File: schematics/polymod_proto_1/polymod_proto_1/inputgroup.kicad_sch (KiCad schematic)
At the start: 10 parts, among them J13 Conn_01x08_Male, U13 74LS165

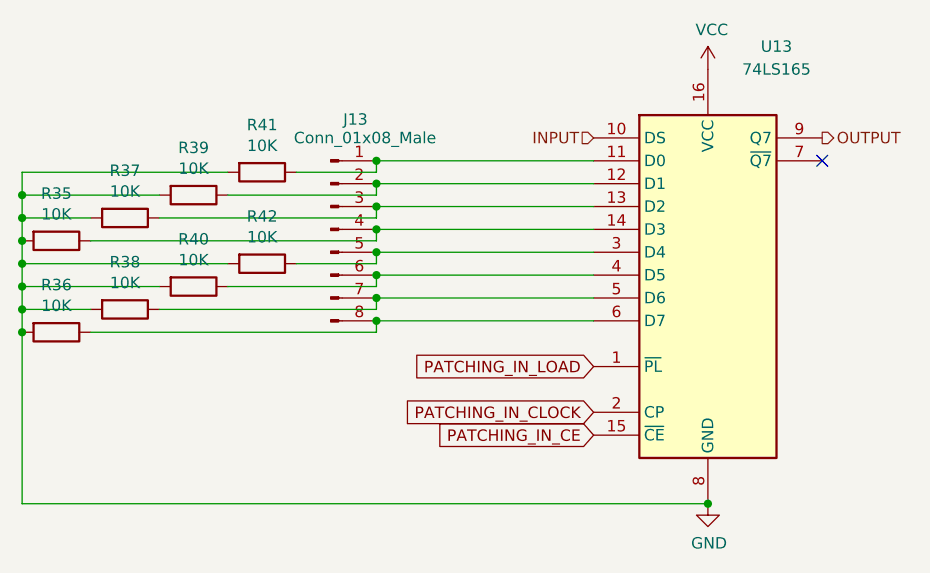
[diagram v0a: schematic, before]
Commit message: routing started
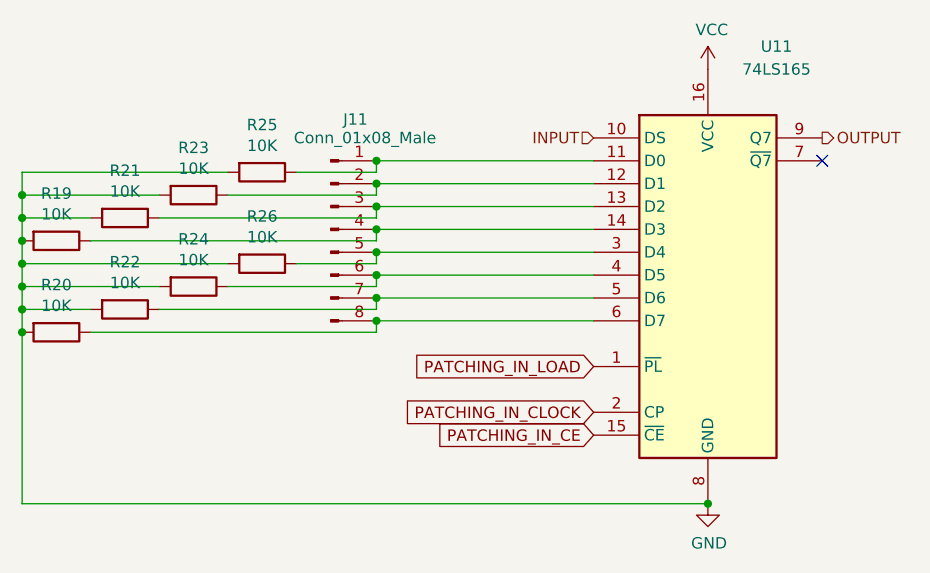
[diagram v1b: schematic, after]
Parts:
- renumbered J13 to J11, R35 to R19, R36 to R20, R37 to R21, R38 to R22, R39 to R23, R40 to R24, R41 to R25, R42 to R26, U13 to U11
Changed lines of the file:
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@@
   (symbol (lib_id "Device:R") (at 118.11 91.44 270)
     (in_bom yes) (on_board yes)
-    (property "Reference" "R40" (id 0) (at 118.11 86.1822 90))
+    (property "Reference" "R24" (id 0) (at 118.11 86.1822 90))
     (property "Value" "10K" (id 1) (at 118.11 88.4936 90))
     (property "Footprint" "Resistor_SMD:R_0805_2012Metric" (id 2) (at 118.11 89.662 90)
@@
   (symbol (lib_id "74xx:74LS165") (at 175.26 90.17 0)
     (in_bom yes) (on_board yes)
-    (property "Reference" "U13" (id 0) (at 182.88 64.77 0))
+    (property "Reference" "U11" (id 0) (at 182.88 64.77 0))
     (property "Value" "74LS165" (id 1) (at 182.88 67.31 0))
     (property "Footprint" "Package_SO:SOIC-16_3.9x9.9mm_P1.27mm" (id 2) (at 175.26 90.17 0)
@@
   (symbol (lib_id "Connector:Conn_01x08_Male") (at 133.35 85.09 0)
     (in_bom yes) (on_board yes)
-    (property "Reference" "J13" (id 0) (at 136.0932 72.8726 0))
+    (property "Reference" "J11" (id 0) (at 136.0932 72.8726 0))
     (property "Value" "Conn_01x08_Male" (id 1) (at 137.16 74.93 0))
     (property "Footprint" "Connector_PinSocket_2.54mm:PinSocket_1x08_P2.54mm_Vertical" (id 2) (at 133.35 85.09 0)
@@
   (symbol (lib_id "power:VCC") (at 175.26 67.31 0)
     (in_bom yes) (on_board yes)
-    (property "Reference" "#PWR030" (id 0) (at 175.26 71.12 0)
+    (property "Reference" "#PWR026" (id 0) (at 175.26 71.12 0)
       (effects (font (size 1.27 1.27)) hide)
     )
@@
   (symbol (lib_id "Device:R") (at 102.87 96.52 270)
     (in_bom yes) (on_board yes)
-    (property "Reference" "R36" (id 0) (at 102.87 91.2622 90))
+    (property "Reference" "R20" (id 0) (at 102.87 91.2622 90))
     (property "Value" "10K" (id 1) (at 102.87 93.5736 90))
     (property "Footprint" "Resistor_SMD:R_0805_2012Metric" (id 2) (at 102.87 94.742 90)
@@
   (symbol (lib_id "Device:R") (at 102.87 86.36 270)
     (in_bom yes) (on_board yes)
-    (property "Reference" "R35" (id 0) (at 102.87 81.1022 90))
+    (property "Reference" "R19" (id 0) (at 102.87 81.1022 90))
     (property "Value" "10K" (id 1) (at 102.87 83.4136 90))
     (property "Footprint" "Resistor_SMD:R_0805_2012Metric" (id 2) (at 102.87 84.582 90)
@@
   (symbol (lib_id "Device:R") (at 118.11 81.28 270)
     (in_bom yes) (on_board yes)
-    (property "Reference" "R39" (id 0) (at 118.11 76.0222 90))
+    (property "Reference" "R23" (id 0) (at 118.11 76.0222 90))
     (property "Value" "10K" (id 1) (at 118.11 78.3336 90))
     (property "Footprint" "Resistor_SMD:R_0805_2012Metric" (id 2) (at 118.11 79.502 90)
@@
   (symbol (lib_id "Device:R") (at 110.49 83.82 270)
     (in_bom yes) (on_board yes)
-    (property "Reference" "R37" (id 0) (at 110.49 78.5622 90))
+    (property "Reference" "R21" (id 0) (at 110.49 78.5622 90))
     (property "Value" "10K" (id 1) (at 110.49 80.8736 90))
     (property "Footprint" "Resistor_SMD:R_0805_2012Metric" (id 2) (at 110.49 82.042 90)
@@
   (symbol (lib_id "Device:R") (at 125.73 88.9 270)
     (in_bom yes) (on_board yes)
-    (property "Reference" "R42" (id 0) (at 125.73 83.6422 90))
+    (property "Reference" "R26" (id 0) (at 125.73 83.6422 90))
     (property "Value" "10K" (id 1) (at 125.73 85.9536 90))
     (property "Footprint" "Resistor_SMD:R_0805_2012Metric" (id 2) (at 125.73 87.122 90)
@@
   (symbol (lib_id "Device:R") (at 125.73 78.74 270)
     (in_bom yes) (on_board yes)
-    (property "Reference" "R41" (id 0) (at 125.73 73.4822 90))
+    (property "Reference" "R25" (id 0) (at 125.73 73.4822 90))
     (property "Value" "10K" (id 1) (at 125.73 75.7936 90))
     (property "Footprint" "Resistor_SMD:R_0805_2012Metric" (id 2) (at 125.73 76.962 90)
@@
   (symbol (lib_id "power:GND") (at 175.26 115.57 0)
     (in_bom yes) (on_board yes)
-    (property "Reference" "#PWR031" (id 0) (at 175.26 121.92 0)
+    (property "Reference" "#PWR027" (id 0) (at 175.26 121.92 0)
       (effects (font (size 1.27 1.27)) hide)
     )
@@
   (symbol (lib_id "Device:R") (at 110.49 93.98 270)
     (in_bom yes) (on_board yes)
-    (property "Reference" "R38" (id 0) (at 110.49 88.7222 90))
+    (property "Reference" "R22" (id 0) (at 110.49 88.7222 90))
     (property "Value" "10K" (id 1) (at 110.49 91.0336 90))
     (property "Footprint" "Resistor_SMD:R_0805_2012Metric" (id 2) (at 110.49 92.202 90)
